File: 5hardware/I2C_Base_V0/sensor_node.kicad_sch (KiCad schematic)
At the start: 57 parts, among them J2 PJ-320D-A, J3 USB_C_Receptacle_USB2.0, J5 Conn_01x15_Pin, P1 S3B-PH-SM4-TB, P3 S3B-PH-SM4-TB, Q1 Si2371EDS, Q2 Si2371EDS, Q3 Si2371EDS, Q5 MMBT5551L, SW3 SW_Push, U12 APDS-9960, U13 SHT31-DIS, U15 DS1307Z+, U16 DS3231M, U17 BH1750FVI-TR, U3 CR2450, U4 CH32V003F4P6, U6 MCP1700x-330xxTO, U7 XC6206PxxxMR, U8 TPL5110, Y1 Crystal, Y2 Crystal

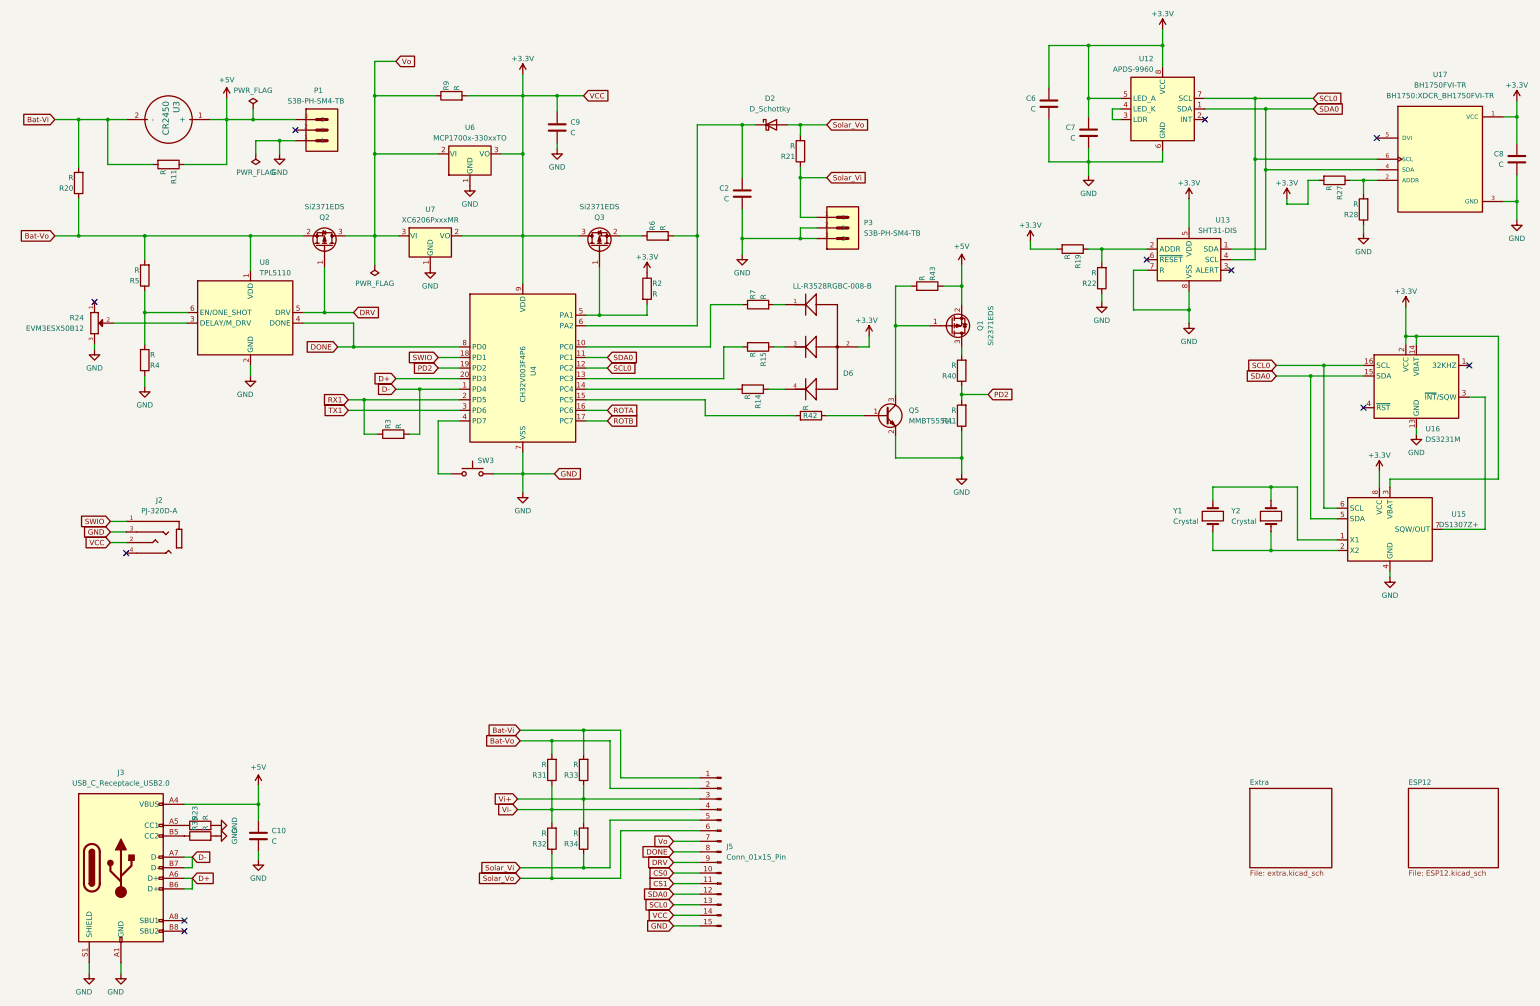
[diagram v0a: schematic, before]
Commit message: update PCB.
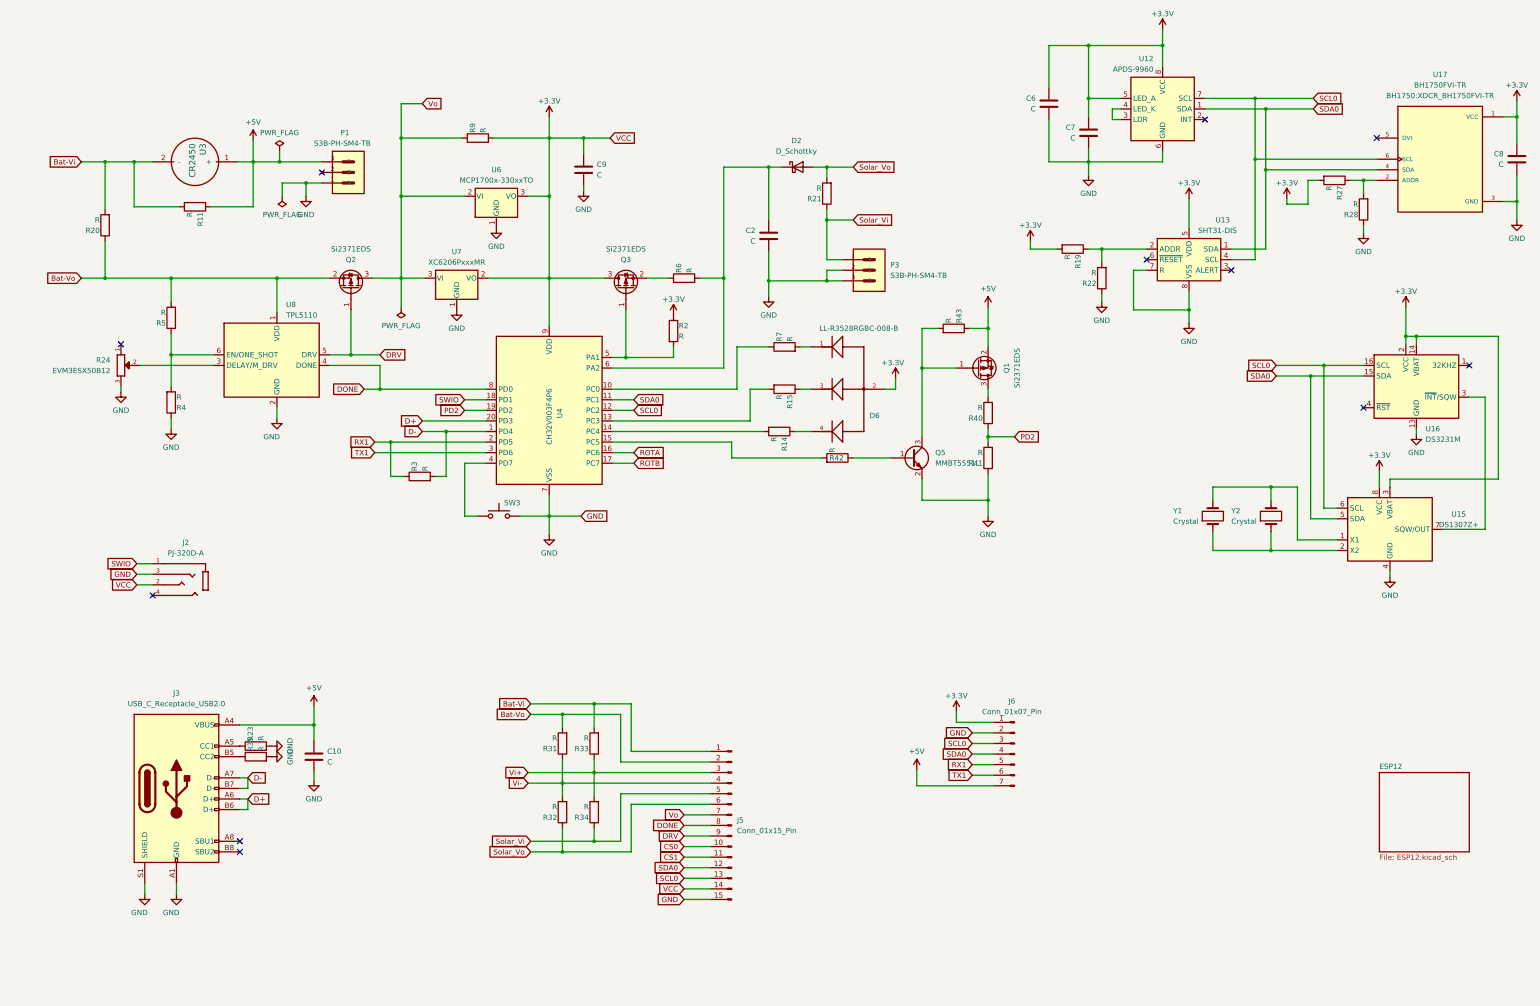
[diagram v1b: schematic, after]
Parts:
- added J6: Conn_01x07_Pin, Connector_PinSocket_2.00mm:PinSocket_1x07_P2.00mm_Vertical, symbol Connector:Conn_01x07_Pin
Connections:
- net +3.3V: now also J6.1 (Pin_1)
- net +5V: now also J6.7 (Pin_7)
- net GND: now also J6.2 (Pin_2)
- net RX1: now also J6.5 (Pin_5)
- net SCL0: now also J6.3 (Pin_3)
- net SDA0: now also J6.4 (Pin_4)
- net TX1: now also J6.6 (Pin_6)
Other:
- removed sheet Extra
- moved on the sheet: C10, C2, C9, D2, D6, J2, J3, J5, P1, P3, Q1, Q2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
